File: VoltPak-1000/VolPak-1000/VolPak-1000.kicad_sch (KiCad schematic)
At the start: 26 parts, among them Y1 40MHz (+/-10PPM)

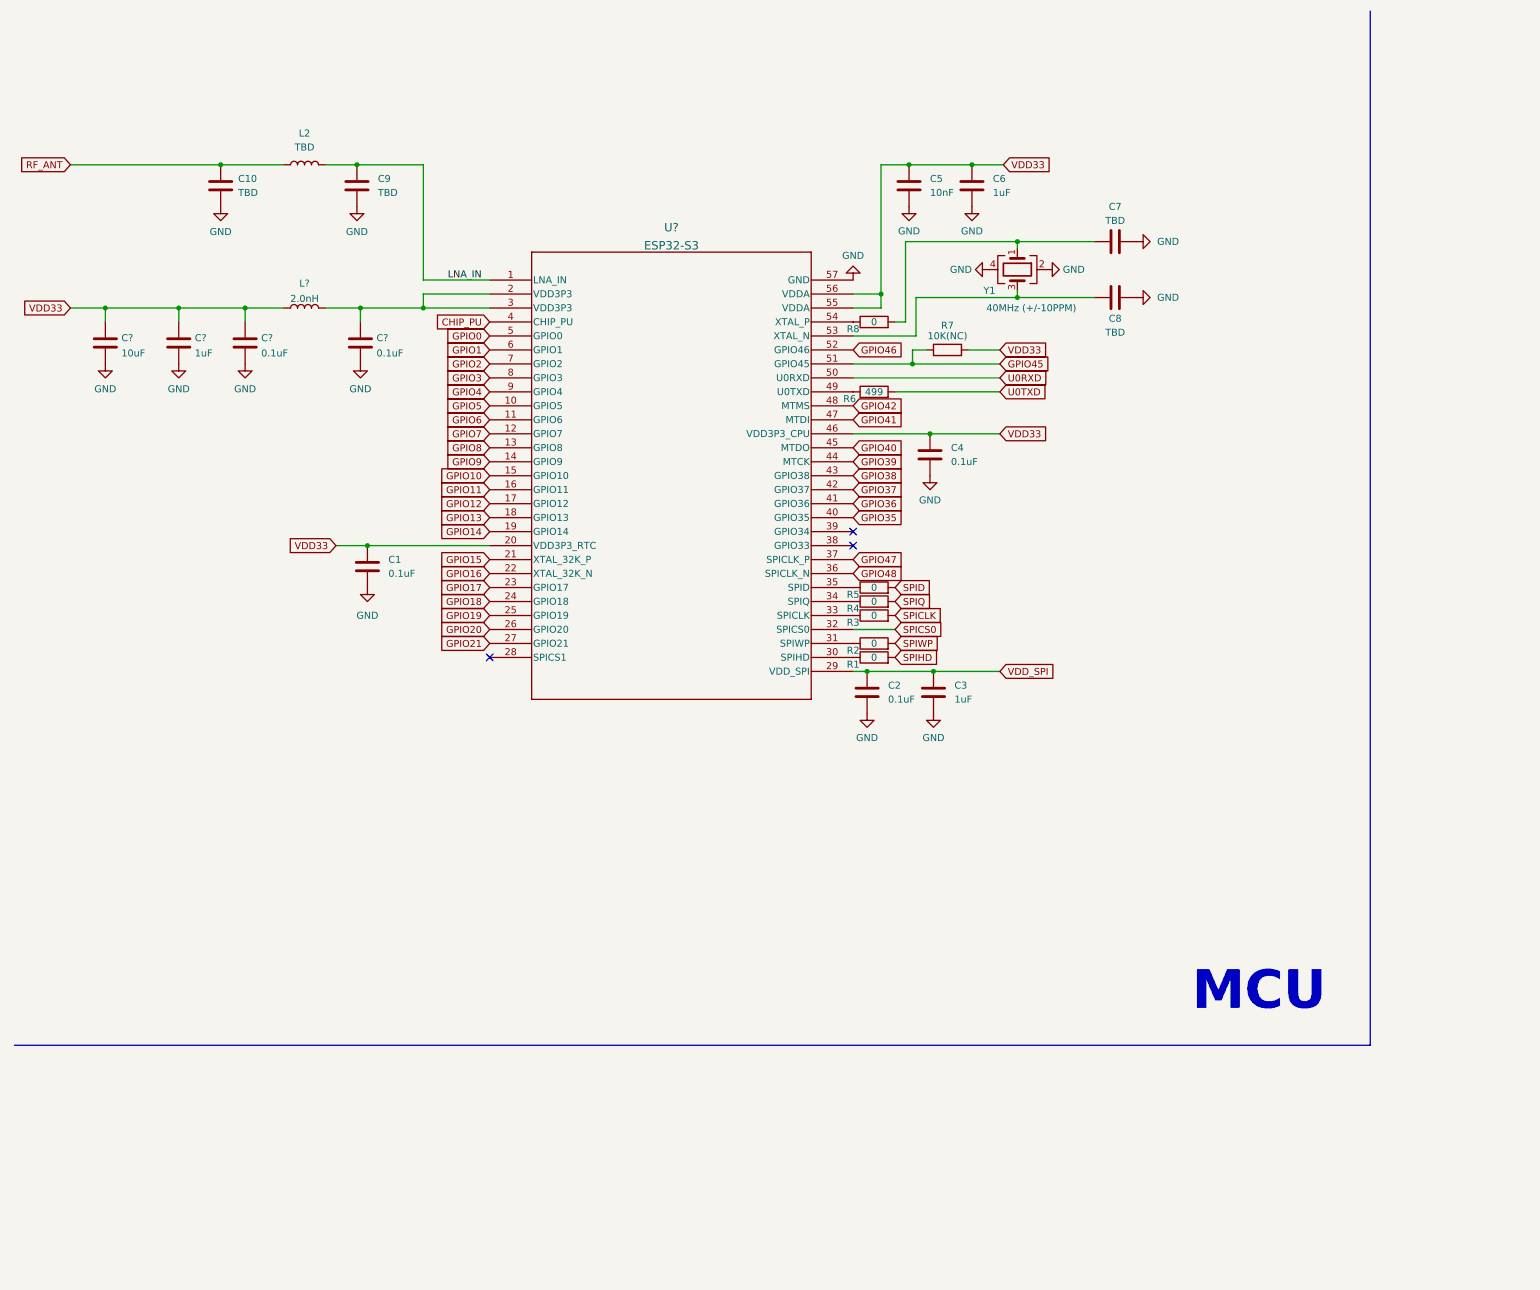
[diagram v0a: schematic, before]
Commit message: almost done mcu
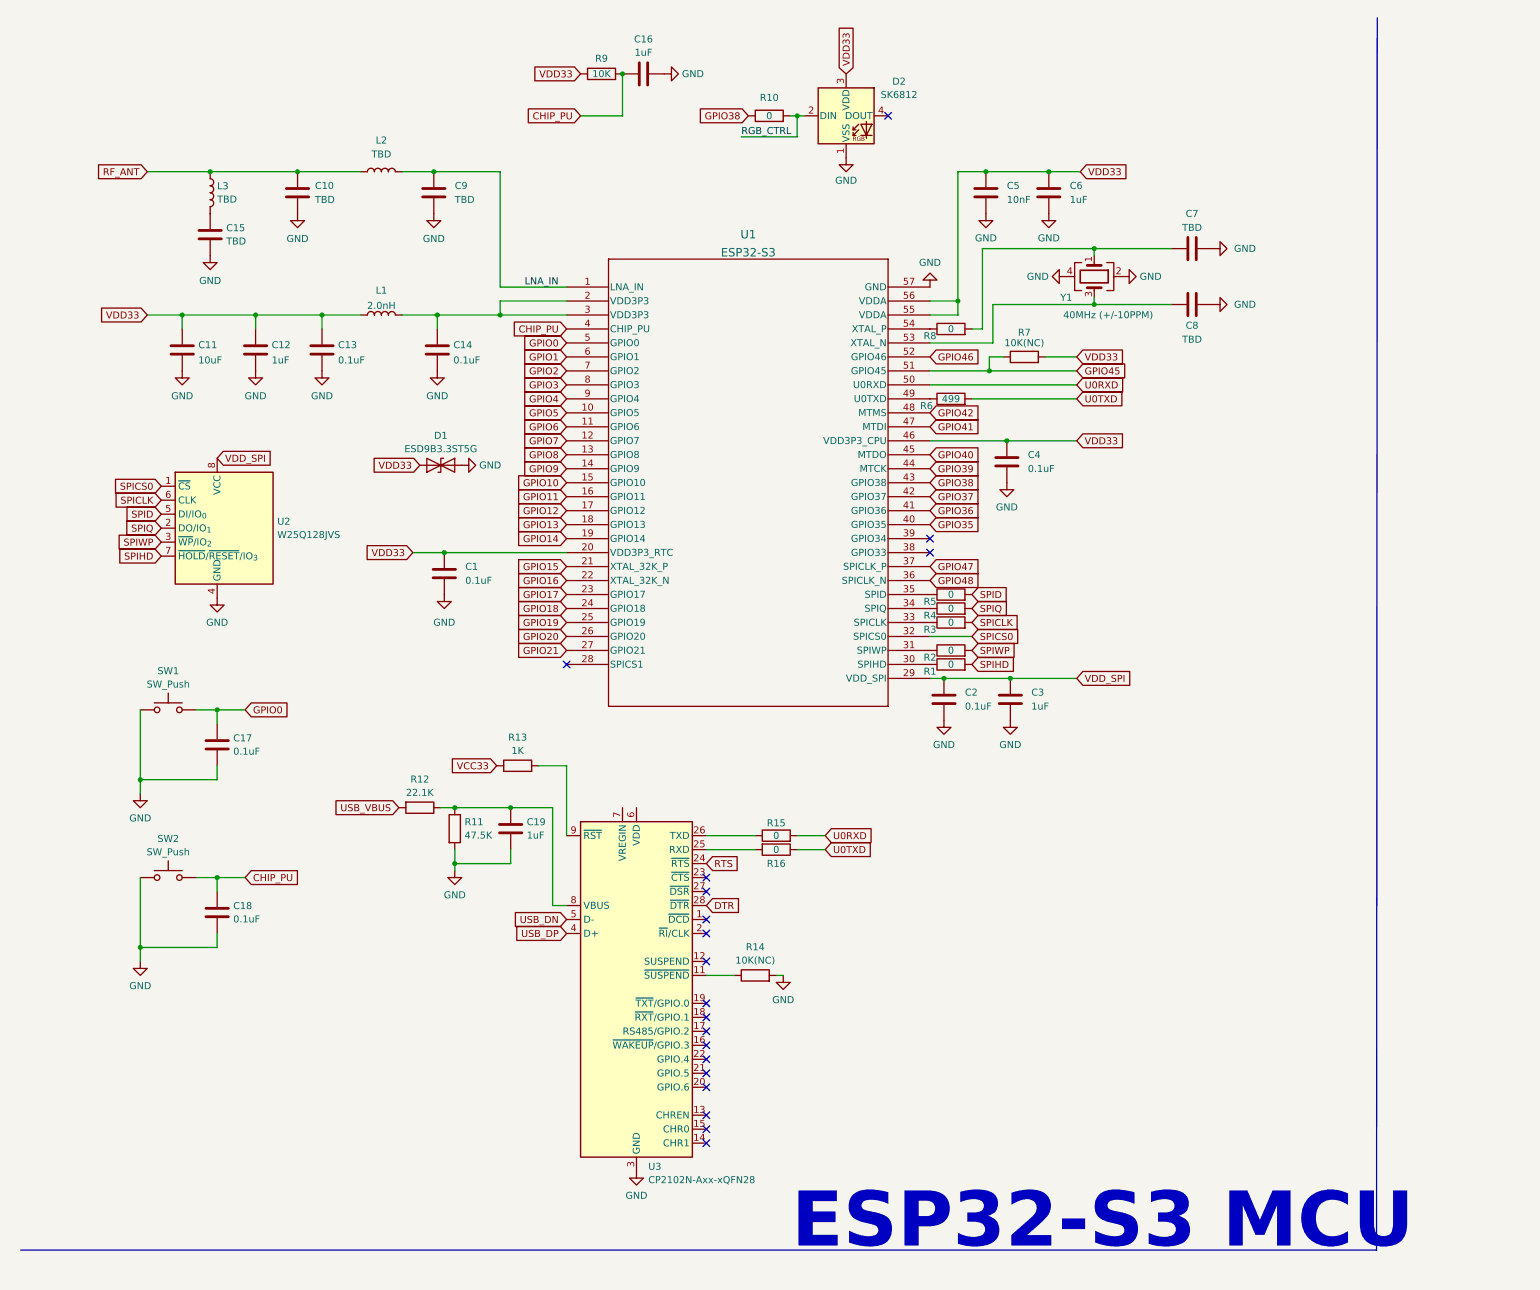
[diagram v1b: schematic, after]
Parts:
- added C15: TBD, symbol Device:C
- added C16, C19: 1uF, symbol Device:C
- added C17, C18: 0.1uF, symbol Device:C
- added D1: ESD9B3.3ST5G, Diode_SMD:D_SOD-923, symbol Diode:ESD9B3.3ST5G
- added D2: SK6812, LED_SMD:LED_SK6812_PLCC4_5.0x5.0mm_P3.2mm, symbol LED:SK6812
- added L3: TBD, symbol Device:L
- added R10, R15, R16: 0, symbol Device:R
- added R11: 47.5K, symbol Device:R
- added R12: 22.1K, symbol Device:R
- added R13: 1K, symbol Device:R
- added R14: 10K(NC), symbol Device:R
- added R9: 10K, symbol Device:R
- added SW1, SW2: SW_Push, symbol Switch:SW_Push
- added U2: W25Q128JVS, Package_SO:SOIC-8_5.3x5.3mm_P1.27mm, symbol Memory_Flash:W25Q128JVS
- added U3: CP2102N-Axx-xQFN28, Package_DFN_QFN:QFN-28-1EP_5x5mm_P0.5mm_EP3.35x3.35mm, symbol Interface_USB:CP2102N-Axx-xQFN28
- gave numbers to parts that had none: 6
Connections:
- net CHIP_PU: now also C16.1, C18.2, R9.2, SW2.2
- net GND: now also C15.2, C16.2, C17.1, C18.1, C19.2, D1.2 (A2), D2.1 (VSS), R11.2, R14.2, SW1.1, SW2.1, U2.4 (GND), U3.29 (GND), U3.3 (GND)
- net GPIO0: now also C17.2, SW1.2
- net GPIO38: now also R10.1
- net RF_ANT: now also L3.1
- net SPICLK: now also U2.6 (CLK)
- net SPICS0: now also U2.1 (~{CS})
- net SPID: now also U2.5 (DI/IO_{0})
- net SPIHD: now also U2.7 (~{HOLD}/~{RESET}/IO_{3})
- net SPIQ: now also U2.2 (DO/IO_{1})
- net SPIWP: now also U2.3 (~{WP}/IO_{2})
- net U0RXD: now also R15.2
- net U0TXD: now also R16.1
- net VDD33: now also D1.1 (A1), D2.3 (VDD), R9.1
- net VDD_SPI: now also U2.8 (VCC)
- new net: R15.1, U3.26 (TXD)
- new net: R14.1, U3.11 (~{SUSPEND})
- new net: R16.2, U3.25 (RXD)
- new net: C19.1, R11.1, R12.1, U3.8 (VBUS)
- new net: R13.2, U3.9 (~{RST})
- new net: C15.1, L3.2
- new net DTR: U3.28 (~{DTR})
- new net RGB_CTRL: D2.2 (DIN), R10.2
- new net RTS: U3.24 (~{RTS})
- new net USB_DN: U3.5 (D-)
- new net USB_DP: U3.4 (D+)
- new net USB_VBUS: R12.2
- new net VCC33: R13.1
- no-connect marks 3 -> 19
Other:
- note added: "ESP32-S3 MCU"
- note removed: "MCU"
- moved on the sheet: C1, C10, C11, C12, C13, C14, C2, C3, C4, C5, C6, C7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
